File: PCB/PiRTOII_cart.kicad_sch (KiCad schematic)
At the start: 10 parts, among them CN1 EDGE_CONN, Q1 BC547, SW1 BTN_RESET_PICO, U1 PICO

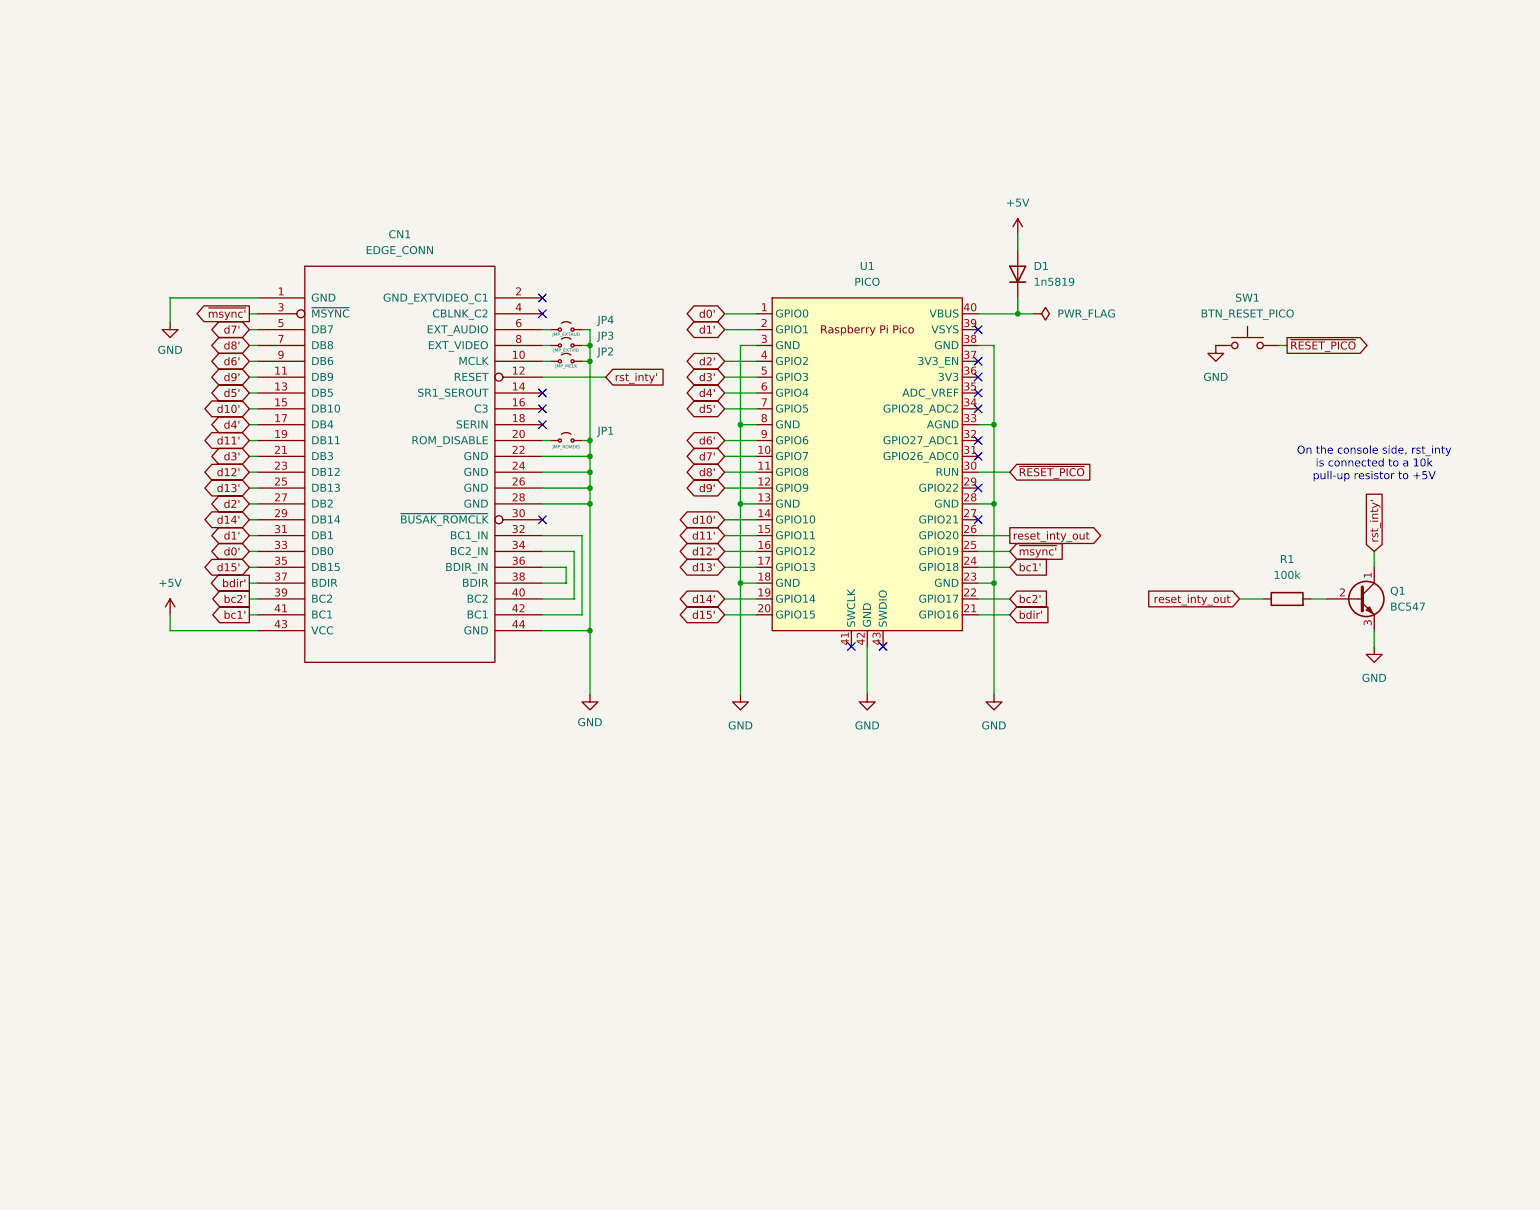
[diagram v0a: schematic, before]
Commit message: Almost there
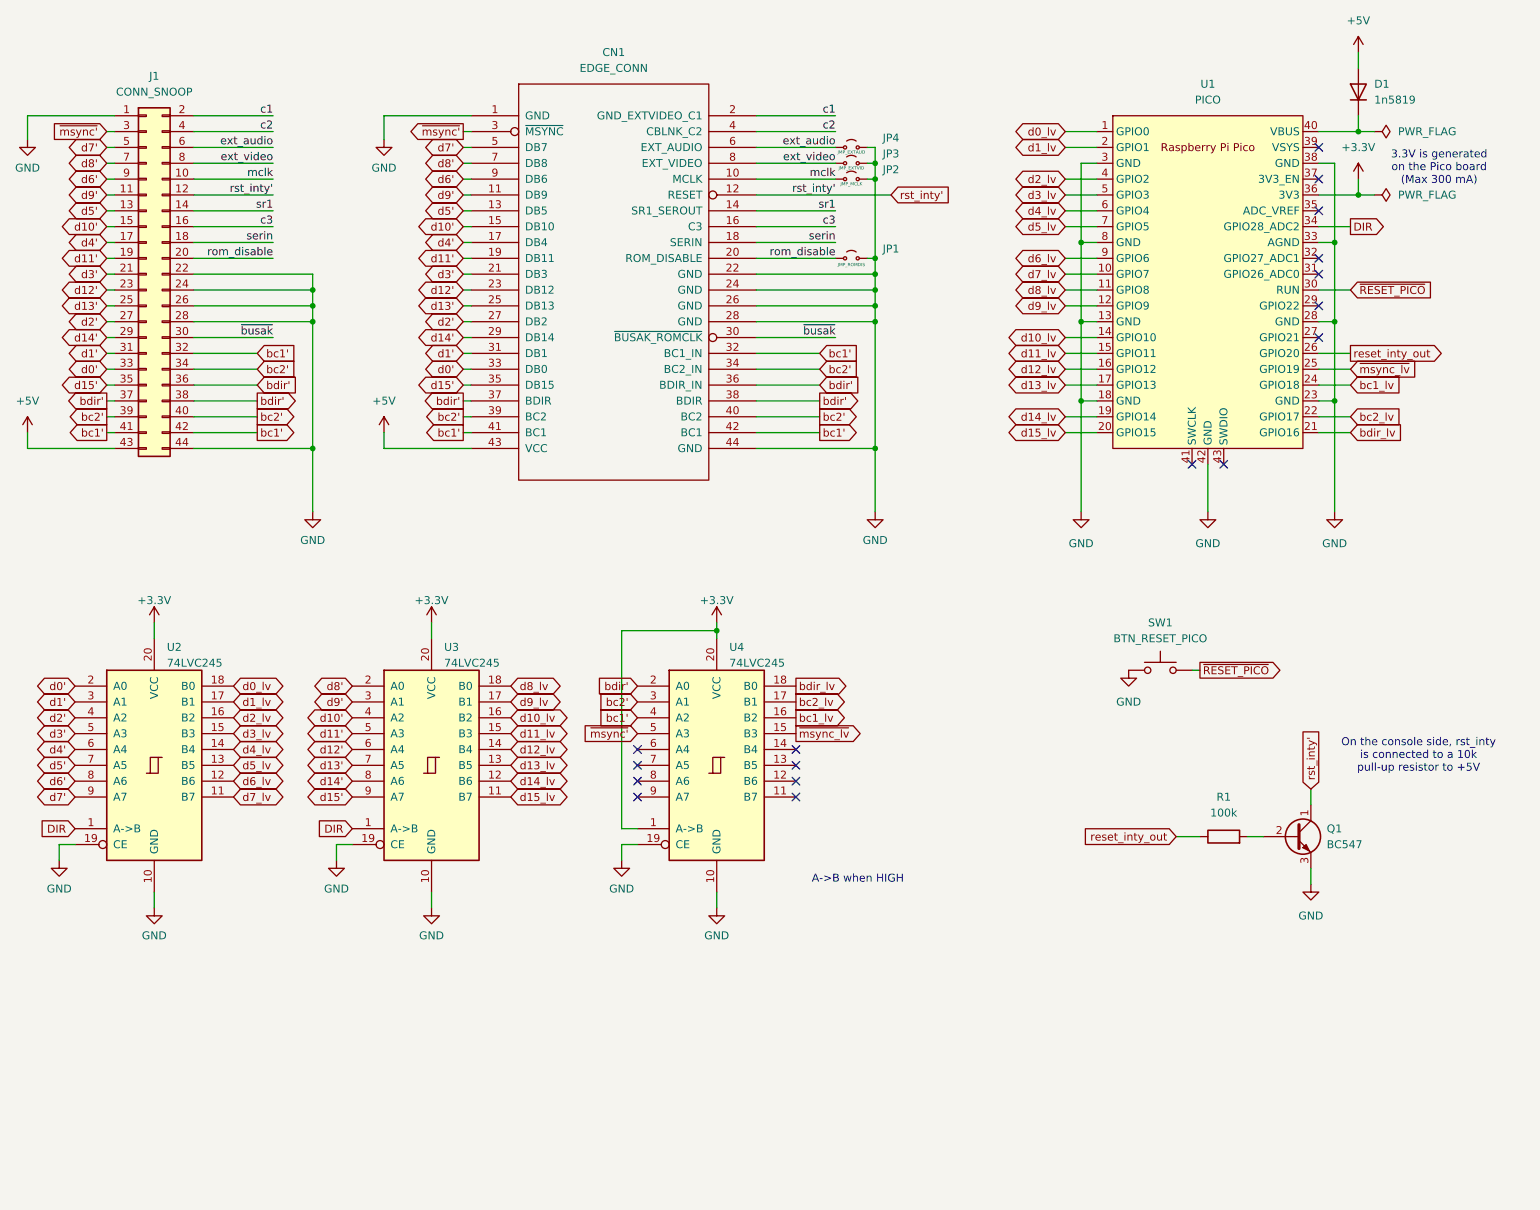
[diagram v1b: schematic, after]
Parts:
- added J1: CONN_SNOOP, Connector_PinHeader_2.54mm:PinHeader_2x22_P2.54mm_Vertical, symbol Connector_Generic:Conn_02x22_Odd_Even
- added U2, U3, U4: 74LVC245, Package_DIP:DIP-20_W7.62mm_Socket_LongPads, symbol 74xx:74LS245
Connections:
- net +5V: now also J1.43 (Pin_43)
- net GND: now also J1.1 (Pin_1), J1.22 (Pin_22), J1.24 (Pin_24), J1.26 (Pin_26), J1.28 (Pin_28), J1.44 (Pin_44), U2.10 (GND), U2.19 (CE), U3.10 (GND), U3.19 (CE), U4.10 (GND), U4.19 (CE)
- net bc1': now also CN1.32 (BC1_IN), CN1.42 (BC1), J1.32 (Pin_32), J1.41 (Pin_41), J1.42 (Pin_42), U4.4 (A2); no longer U1.24 (GPIO18)
- net bc2': now also CN1.34 (BC2_IN), CN1.40 (BC2), J1.34 (Pin_34), J1.39 (Pin_39), J1.40 (Pin_40), U4.3 (A1); no longer U1.22 (GPIO17)
- net bdir': now also CN1.36 (BDIR_IN), CN1.38 (BDIR), J1.36 (Pin_36), J1.37 (Pin_37), J1.38 (Pin_38), U4.2 (A0); no longer U1.21 (GPIO16)
- net d0': now also J1.33 (Pin_33), U2.2 (A0); no longer U1.1 (GPIO0)
- net d1': now also J1.31 (Pin_31), U2.3 (A1); no longer U1.2 (GPIO1)
- net d10': now also J1.15 (Pin_15), U3.4 (A2); no longer U1.14 (GPIO10)
- net d11': now also J1.19 (Pin_19), U3.5 (A3); no longer U1.15 (GPIO11)
- net d12': now also J1.23 (Pin_23), U3.6 (A4); no longer U1.16 (GPIO12)
- net d13': now also J1.25 (Pin_25), U3.7 (A5); no longer U1.17 (GPIO13)
- net d14': now also J1.29 (Pin_29), U3.8 (A6); no longer U1.19 (GPIO14)
- net d15': now also J1.35 (Pin_35), U3.9 (A7); no longer U1.20 (GPIO15)
- net d2': now also J1.27 (Pin_27), U2.4 (A2); no longer U1.4 (GPIO2)
- net d3': now also J1.21 (Pin_21), U2.5 (A3); no longer U1.5 (GPIO3)
- net d4': now also J1.17 (Pin_17), U2.6 (A4); no longer U1.6 (GPIO4)
- net d5': now also J1.13 (Pin_13), U2.7 (A5); no longer U1.7 (GPIO5)
- net d6': now also J1.9 (Pin_9), U2.8 (A6); no longer U1.9 (GPIO6)
- net d7': now also J1.5 (Pin_5), U2.9 (A7); no longer U1.10 (GPIO7)
- net d8': now also J1.7 (Pin_7), U3.2 (A0); no longer U1.11 (GPIO8)
- net d9': now also J1.11 (Pin_11), U3.3 (A1); no longer U1.12 (GPIO9)
- net rst_inty': now also J1.12 (Pin_12)
- net ~{msync'}: now also J1.3 (Pin_3), U4.5 (A3); no longer U1.25 (GPIO19)
- net ext_audio: now reaches CN1.6 (EXT_AUDIO), JP4.1 (A)
- net ext_audio: now also J1.6 (Pin_6)
- net DIR: now reaches U1.34 (GPIO28_ADC2)
- net DIR: now also U2.1 (A->B), U3.1 (A->B)
- net +3.3V: now reaches U1.36 (3V3)
- net +3.3V: now also U2.20 (VCC), U3.20 (VCC), U4.1 (A->B), U4.20 (VCC)
- net ext_video: now reaches CN1.8 (EXT_VIDEO), JP3.1 (A)
- net ext_video: now also J1.8 (Pin_8)
- net mclk: now reaches CN1.10 (MCLK), JP2.1 (A)
- net mclk: now also J1.10 (Pin_10)
- net sr1: now reaches CN1.14 (SR1_SEROUT)
- net sr1: now also J1.14 (Pin_14)
- net c3: now reaches CN1.16 (C3)
- net c3: now also J1.16 (Pin_16)
- net serin: now reaches CN1.18 (SERIN)
- net serin: now also J1.18 (Pin_18)
- net c1: now reaches CN1.2 (GND_EXTVIDEO_C1)
- net c1: now also J1.2 (Pin_2)
- net rom_disable: now reaches CN1.20 (ROM_DISABLE), JP1.1 (A)
- net rom_disable: now also J1.20 (Pin_20)
- net ~{busak}: now reaches CN1.30 (~{BUSAK_ROMCLK})
- net ~{busak}: now also J1.30 (Pin_30)
- net c2: now reaches CN1.4 (CBLNK_C2)
- net c2: now also J1.4 (Pin_4)
- new net bc1_lv: U1.24 (GPIO18), U4.16 (B2)
- new net bc2_lv: U1.22 (GPIO17), U4.17 (B1)
- new net bdir_lv: U1.21 (GPIO16), U4.18 (B0)
- new net d0_lv: U1.1 (GPIO0), U2.18 (B0)
- new net d10_lv: U1.14 (GPIO10), U3.16 (B2)
- new net d11_lv: U1.15 (GPIO11), U3.15 (B3)
- new net d12_lv: U1.16 (GPIO12), U3.14 (B4)
- new net d13_lv: U1.17 (GPIO13), U3.13 (B5)
- new net d14_lv: U1.19 (GPIO14), U3.12 (B6)
- new net d15_lv: U1.20 (GPIO15), U3.11 (B7)
- new net d1_lv: U1.2 (GPIO1), U2.17 (B1)
- new net d2_lv: U1.4 (GPIO2), U2.16 (B2)
- new net d3_lv: U1.5 (GPIO3), U2.15 (B3)
- new net d4_lv: U1.6 (GPIO4), U2.14 (B4)
- new net d5_lv: U1.7 (GPIO5), U2.13 (B5)
- new net d6_lv: U1.9 (GPIO6), U2.12 (B6)
- new net d7_lv: U1.10 (GPIO7), U2.11 (B7)
- new net d8_lv: U1.11 (GPIO8), U3.18 (B0)
- new net d9_lv: U1.12 (GPIO9), U3.17 (B1)
- new net ~{msync_lv}: U1.25 (GPIO19), U4.15 (B3)
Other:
- note added: "3.3V is generated on the Pico board (Max 300 mA)"
- note added: "A->B when HIGH"
- company: Andrea Ottaviani -> Andrea Ottaviani/SukkoPera
- title: RTO-Multicart -> PiRTO II Cart - "Official Pico" Edition
- moved on the sheet: CN1, D1, JP1, JP2, JP3, JP4, Q1, R1, SW1, U1

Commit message: Add MicroSD slot
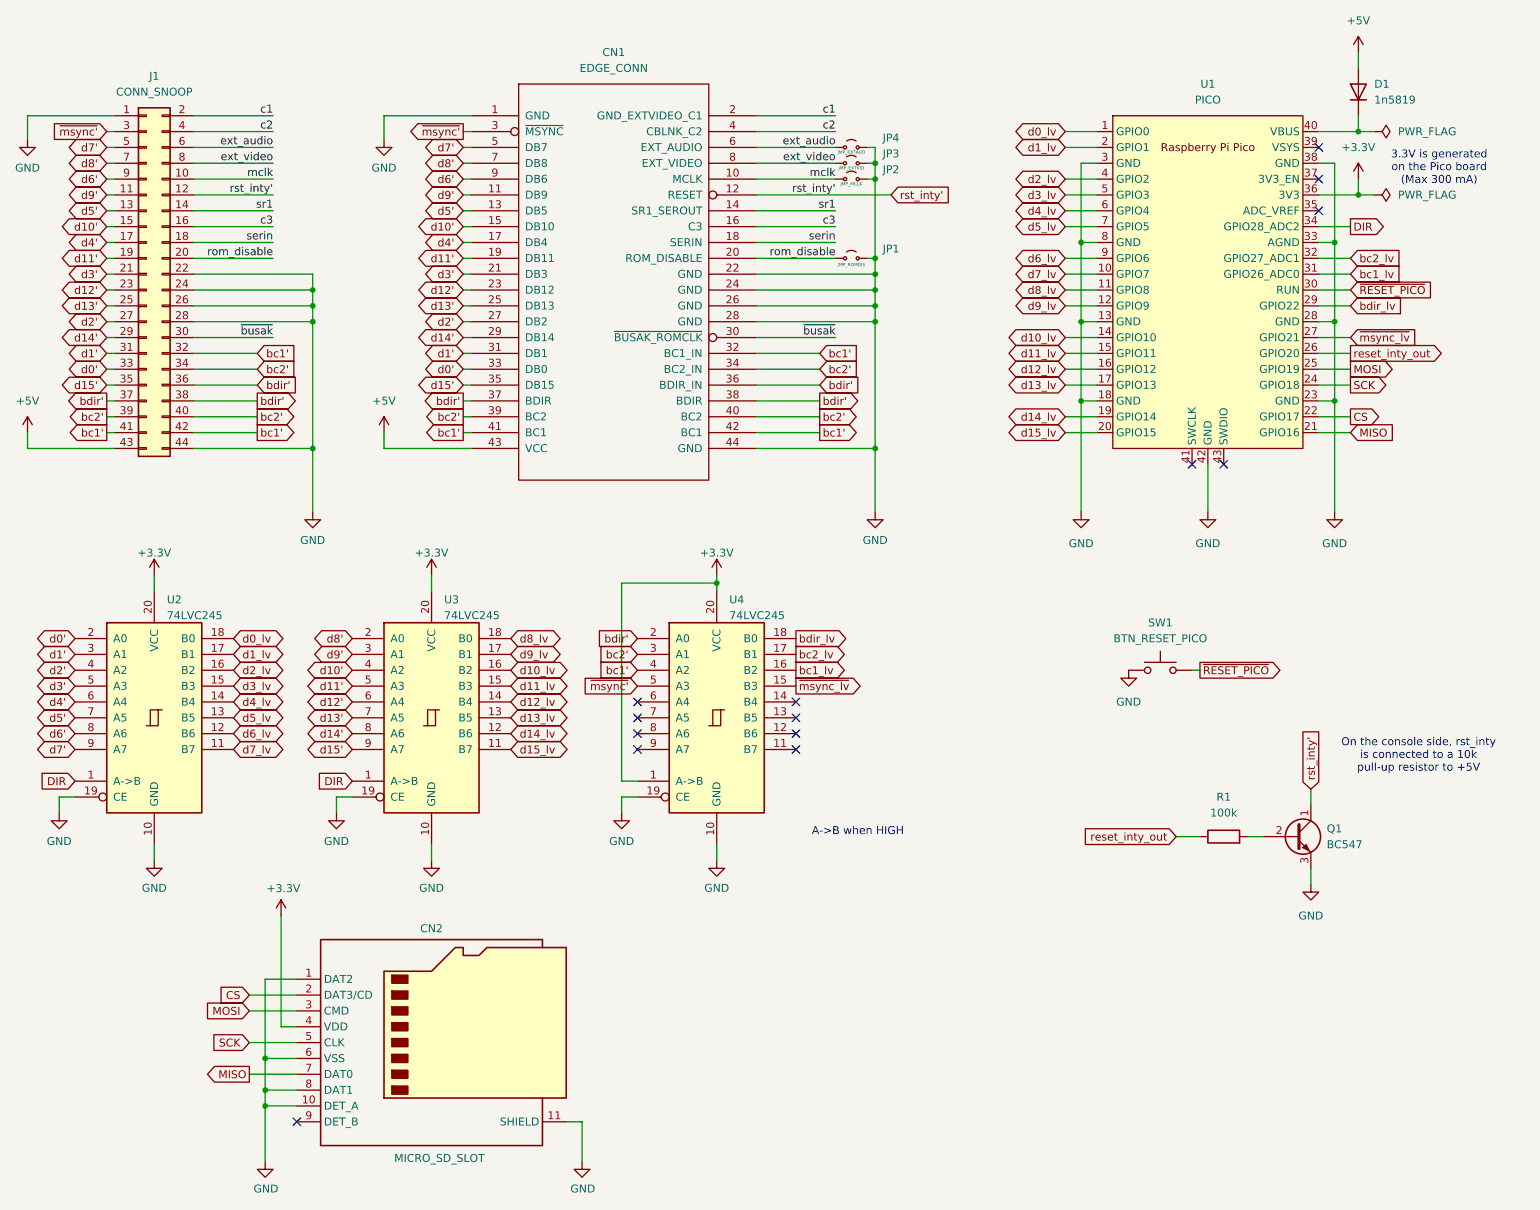
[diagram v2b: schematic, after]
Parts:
- added CN2: MICRO_SD_SLOT, PiRTOII:GCT-MEM2055-00-190-01-A, symbol Connector:Micro_SD_Card_Det2
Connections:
- net +3.3V: now also CN2.4 (VDD)
- net GND: now also CN2.1 (DAT2), CN2.10 (DET_A), CN2.11 (SHIELD), CN2.6 (VSS), CN2.8 (DAT1)
- net bc1_lv: now also U1.31 (GPIO26_ADC0); no longer U1.24 (GPIO18)
- net bc2_lv: now also U1.32 (GPIO27_ADC1); no longer U1.22 (GPIO17)
- net bdir_lv: now also U1.29 (GPIO22); no longer U1.21 (GPIO16)
- net ~{msync_lv}: now also U1.27 (GPIO21); no longer U1.25 (GPIO19)
- new net CS: CN2.2 (DAT3/CD), U1.22 (GPIO17)
- new net MISO: CN2.7 (DAT0), U1.21 (GPIO16)
- new net MOSI: CN2.3 (CMD), U1.25 (GPIO19)
- new net SCK: CN2.5 (CLK), U1.24 (GPIO18)
- no-connect marks 17 -> 14
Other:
- moved on the sheet: U2, U3, U4
